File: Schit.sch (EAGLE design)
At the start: 15 parts, among them IC2 MEGA16-A, Q1 12M

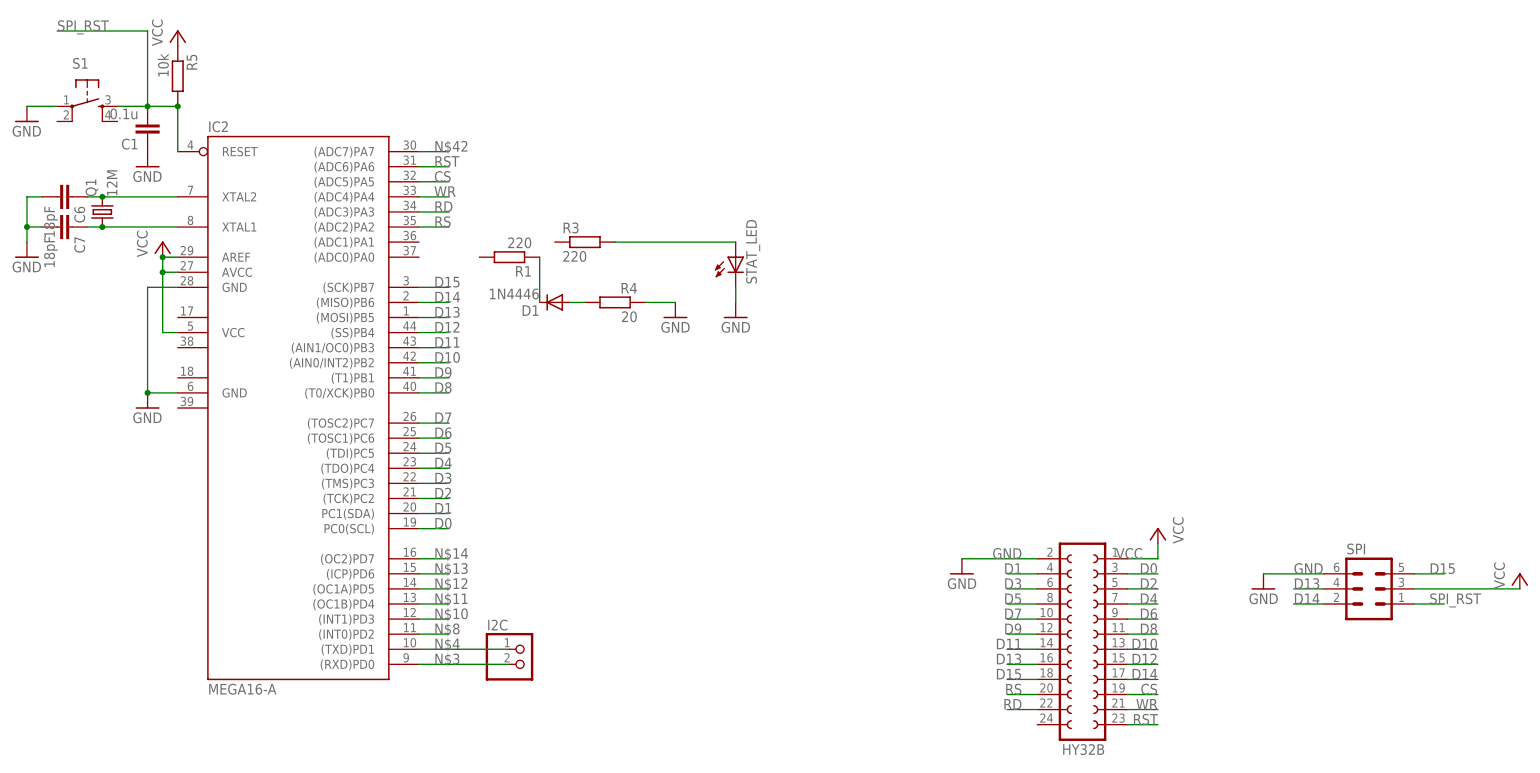
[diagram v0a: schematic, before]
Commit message: 1.0.1
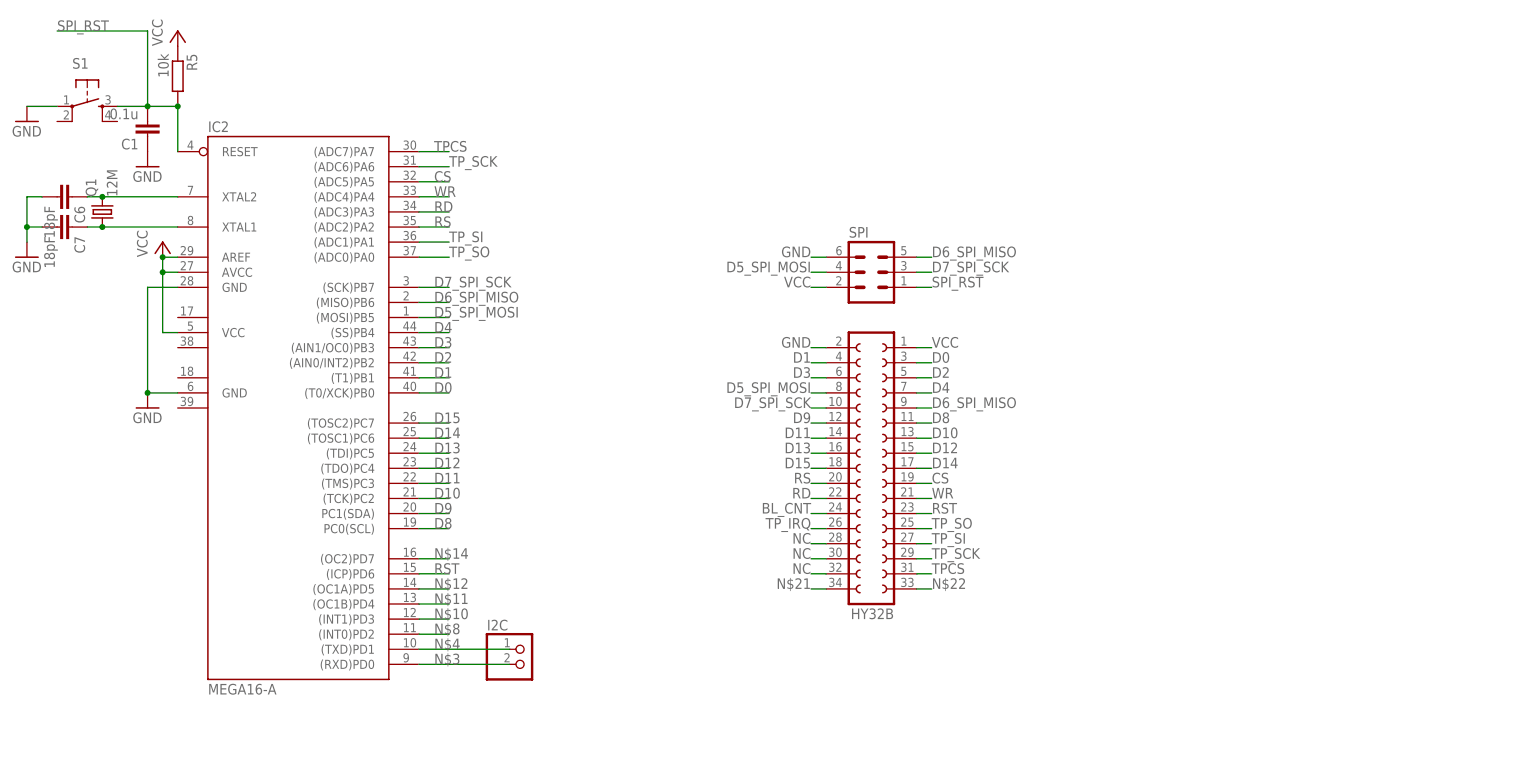
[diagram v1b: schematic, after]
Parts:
- removed D1: 1N4446, diode:1N4446
- removed R1: 220, resistor:R-EU_R1206
- removed R3: 220, rcl:R-EU_M2012
- removed R4: 20, resistor:R-EU_R1206
- removed STAT_LED: (no value), led:LED3MM
- HY32B: device con-lsta:FE12-2 -> con-lsta:FE17-2
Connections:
- removed net D5: HY32B.8, IC2.(TDI)PC5
- removed net D6: HY32B.9, IC2.(TOSC1)PC6
- removed net D7: HY32B.10, IC2.(TOSC2)PC7
- removed net N$1: D1.C, R1.1
- removed net N$13: IC2.(ICP)PD6
- removed net N$2: D1.A, R4.2
- removed net N$42: IC2.(ADC7)PA7
- removed net N$9: R3.2, STAT_LED.A
- new net BL_CNT: HY32B.24
- new net D5_SPI_MOSI: HY32B.8, IC2.(MOSI)PB5, SPI.4
- new net D6_SPI_MISO: HY32B.9, IC2.(MISO)PB6, SPI.5
- new net D7_SPI_SCK: HY32B.10, IC2.(SCK)PB7, SPI.3
- new net N$21: HY32B.34
- new net N$22: HY32B.33
- new net NC: HY32B.28, HY32B.30, HY32B.32
- new net TPCS: HY32B.31, IC2.(ADC7)PA7
- new net TP_IRQ: HY32B.26
- new net TP_SCK: HY32B.29, IC2.(ADC6)PA6
- new net TP_SI: HY32B.27, IC2.(ADC1)PA1
- new net TP_SO: HY32B.25, IC2.(ADC0)PA0
- net D0: now also IC2.(T0/XCK)PB0; no longer IC2.PC0(SCL)
- net D1: now also IC2.(T1)PB1; no longer IC2.PC1(SDA)
- net D10: now also IC2.(TCK)PC2; no longer IC2.(AIN0/INT2)PB2
- net D11: now also IC2.(TMS)PC3; no longer IC2.(AIN1/OC0)PB3
- net D12: now also IC2.(TDO)PC4; no longer IC2.(SS)PB4
- net D13: now also IC2.(TDI)PC5; no longer IC2.(MOSI)PB5, SPI.4
- net D14: now also IC2.(TOSC1)PC6; no longer IC2.(MISO)PB6, SPI.2
- net D15: now also IC2.(TOSC2)PC7; no longer IC2.(SCK)PB7, SPI.5
- net D2: now also IC2.(AIN0/INT2)PB2; no longer IC2.(TCK)PC2
- net D3: now also IC2.(AIN1/OC0)PB3; no longer IC2.(TMS)PC3
- net D4: now also IC2.(SS)PB4; no longer IC2.(TDO)PC4
- net D8: now also IC2.PC0(SCL); no longer IC2.(T0/XCK)PB0
- net D9: now also IC2.PC1(SDA); no longer IC2.(T1)PB1
- net GND: no longer R4.1, STAT_LED.C
- net RST: now also IC2.(ICP)PD6; no longer IC2.(ADC6)PA6
- net VCC: now also SPI.2; no longer SPI.3
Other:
- moved on the sheet: SPI
